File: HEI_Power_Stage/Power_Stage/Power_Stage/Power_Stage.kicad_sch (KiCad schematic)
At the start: 1 part, among them Q1 EPC2304ENGRT

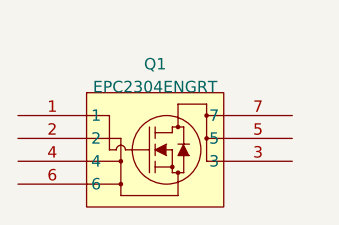
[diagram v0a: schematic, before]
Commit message: second try for kicad libs
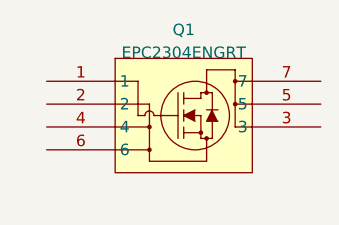
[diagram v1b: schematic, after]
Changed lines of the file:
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@@
 (kicad_sch (version 20230121) (generator eeschema)
   (paper "A4")
-  (symbol (lib_id "GTSR_symbol_lib_SD:EPC2304ENGRT") (at 150.495 96.52 0) (unit 1)
+  (symbol (lib_id "GTSR_symbol_lib_SD:EPC2304ENGRT") (at 153.67 92.71 0) (unit 1)
     (in_bom yes) (on_board yes) (dnp no) (fields_autoplaced)
-    (property "Reference" "Q1" (at 150.495 95.25 0)
+    (property "Reference" "Q1" (at 153.67 91.44 0)
       (effects (font (size 1.27 1.27)))
     )
-    (property "Value" "EPC2304ENGRT" (at 150.495 97.79 0)
+    (property "Value" "EPC2304ENGRT" (at 153.67 93.98 0)
       (effects (font (size 1.27 1.27)))
     )
-    (property "Footprint" "GTSR_KiCAD_Footprints_SD:EPC2304_ECC" (at 150.495 96.52 0)
+    (property "Footprint" "GTSR_KiCAD_Footprints_SD:EPC2304_ECC" (at 153.67 92.71 0)
       (effects (font (size 1.27 1.27)) hide)
     )
-    (property "Datasheet" "https://www.digikey.com/en/products/detail/epc/EPC2304ENGRT/16785484" (at 150.495 96.52 0)
+    (property "Datasheet" "https://www.digikey.com/en/products/detail/epc/EPC2304ENGRT/16785484" (at 153.67 92.71 0)
       (effects (font (size 1.27 1.27)) hide)
     )
